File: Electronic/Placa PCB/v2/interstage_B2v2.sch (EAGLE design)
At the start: 7 parts, among them P1 0532610271, Q1 PMV16XNR, U1 MCP9808T-E/MS, U3 MCP9808T-E/MS

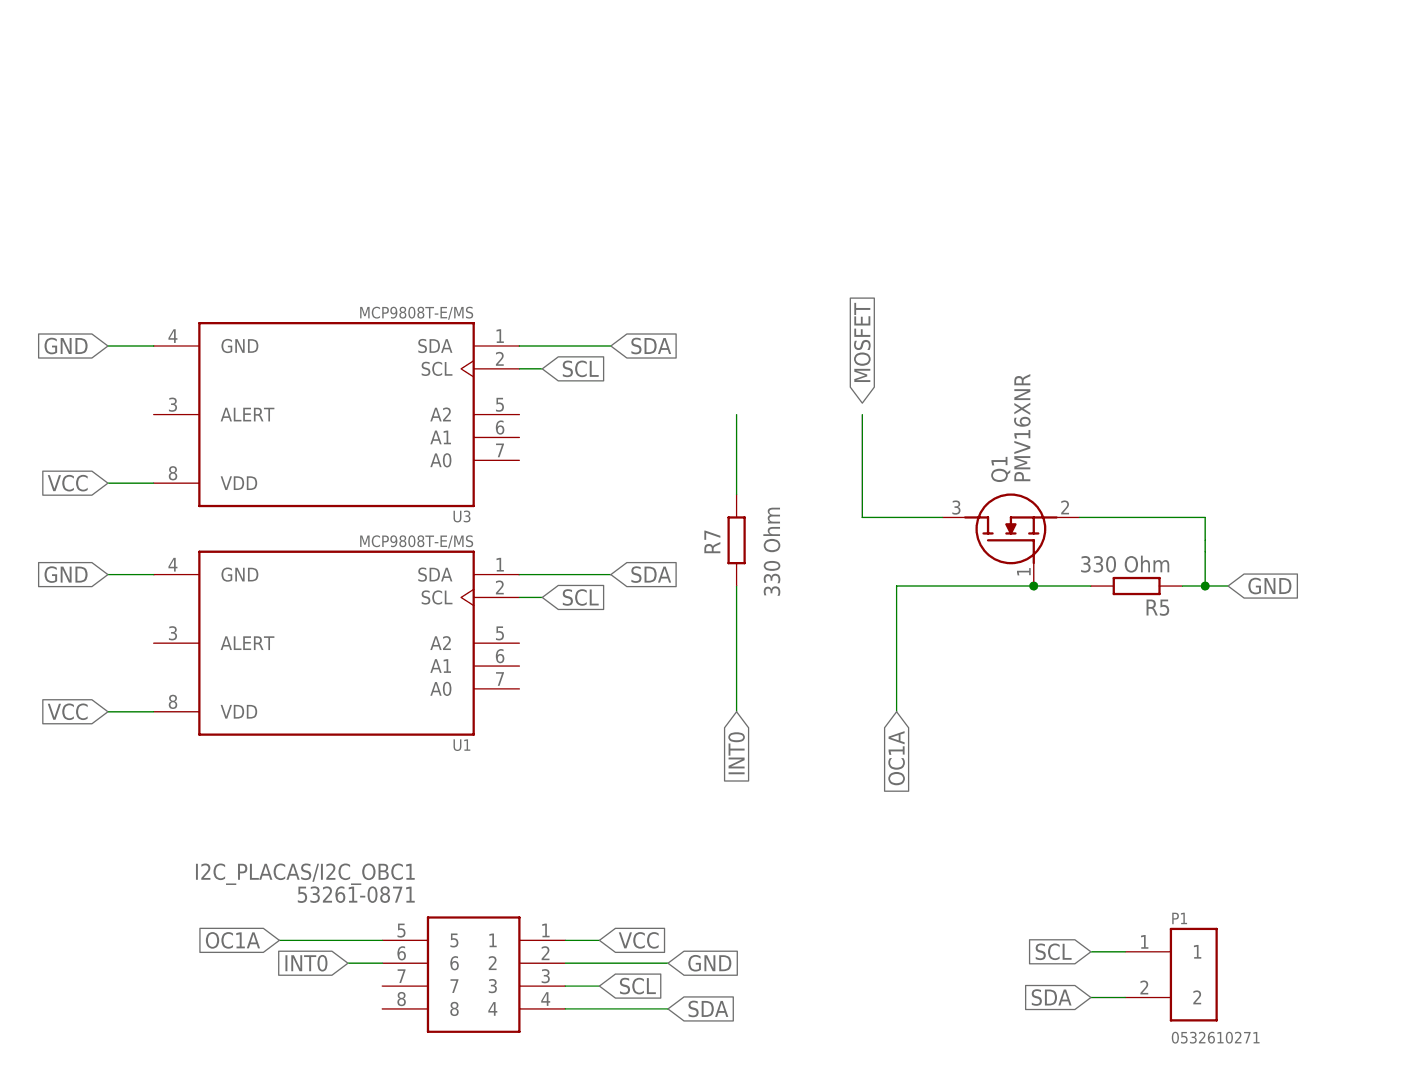
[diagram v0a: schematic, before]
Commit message: Placas PCB
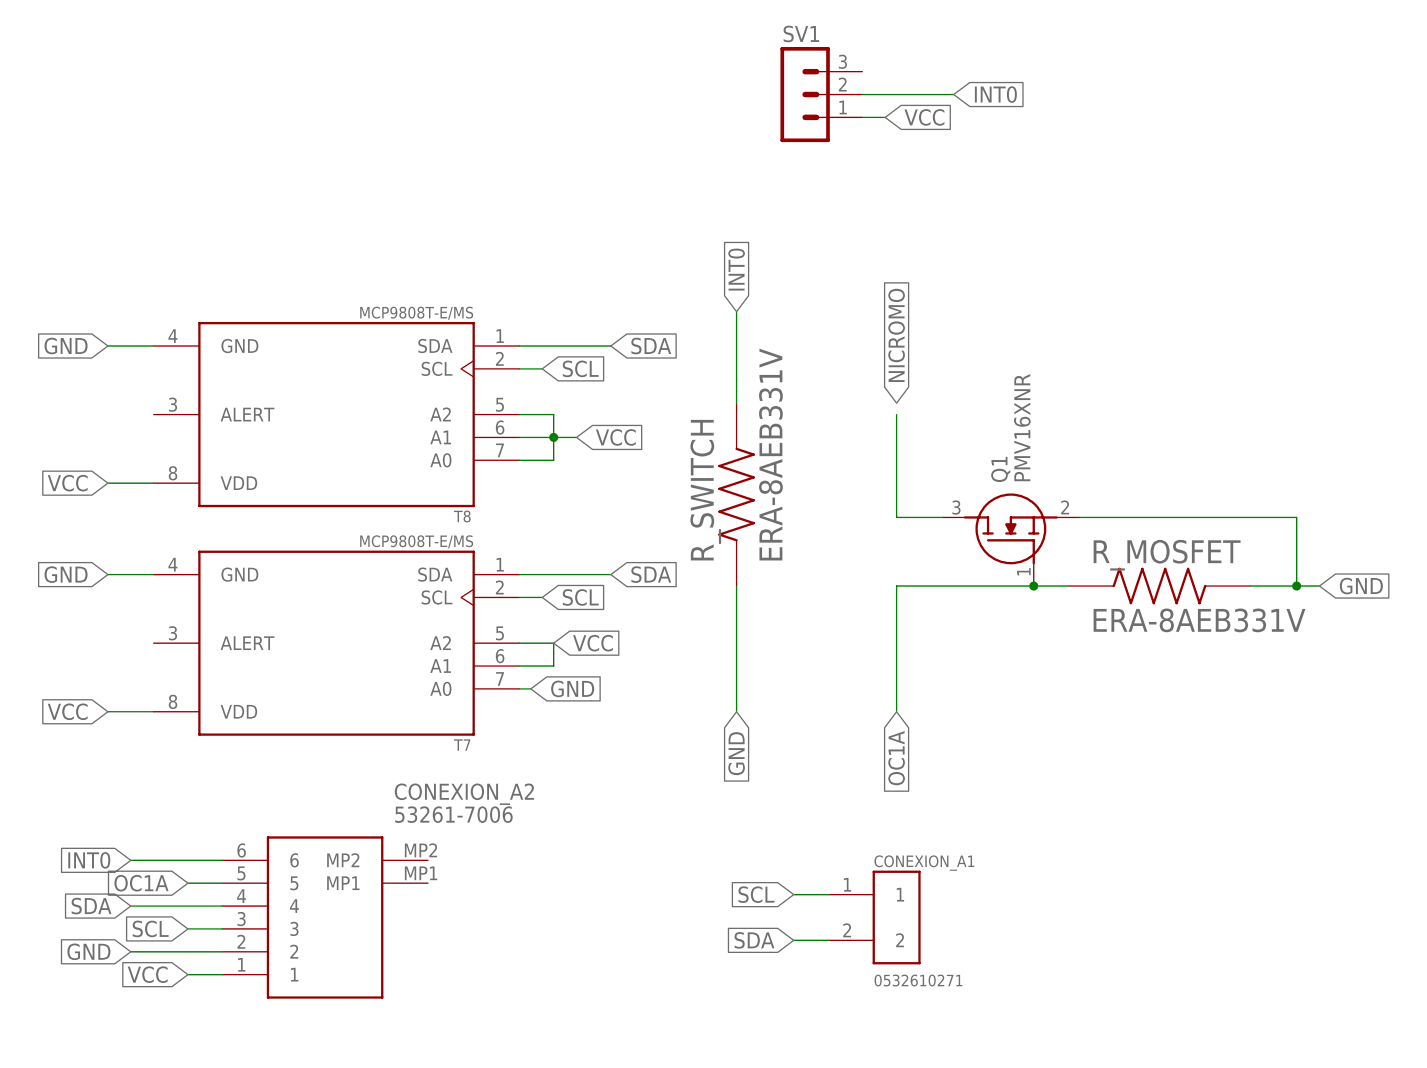
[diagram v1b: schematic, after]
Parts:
- removed I2C_PLACAS/I2C_OBC1: 53261-0871, SamacSys_Parts:53261-0871
- removed P1: 0532610271, picoblade2:0532610271
- removed R5, R7: 330 Ohm, rcl:R-EU_R1206
- added CONEXION_A1: 0532610271, picoblade2:0532610271
- added CONEXION_A2: 53261-7006, SamacSys_Parts:53261-7006
- added R_MOSFET, R_SWITCH: ERA-8AEB331V, resistor_330_smd:ERA-8AEB331V
- added SV1: (no value), con-lstb:MA03-1
- renumbered U1 to T7, U3 to T8
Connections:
- net MOSFET renamed NICROMO
- removed net N$1: R7.1
- net GND: now also CONEXION_A2.2, R_MOSFET.2, R_SWITCH.1, T7.A0; no longer I2C_PLACAS/I2C_OBC1.2, R5.1
- net INT0: now also CONEXION_A2.6, R_SWITCH.2, SV1.2; no longer I2C_PLACAS/I2C_OBC1.6, R7.2
- net OC1A: now also CONEXION_A2.5, R_MOSFET.1; no longer I2C_PLACAS/I2C_OBC1.5, R5.2
- net SCL: now also CONEXION_A1.1, CONEXION_A2.3; no longer I2C_PLACAS/I2C_OBC1.3, P1.1
- net SDA: now also CONEXION_A1.2, CONEXION_A2.4; no longer I2C_PLACAS/I2C_OBC1.4, P1.2
- net VCC: now also CONEXION_A2.1, SV1.1, T7.A1, T7.A2, T8.A0, T8.A1, T8.A2; no longer I2C_PLACAS/I2C_OBC1.1
